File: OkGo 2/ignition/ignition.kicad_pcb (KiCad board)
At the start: 2 copper layers, 100 parts, among them K201 16A SPST, K202 16A SPST, K203 16A SPST, K204 16A SPST, K205 16A SPST, P105 BATT, P106 SMA, P107 ARM_LED, P109 BUZZ, P201 CH3_LED, P203 CH3, P204 CH1_LED, P206 CH1, P207 CH4_LED, P209 CH4, P210 CH2_LED, P212 CH2, Q101 BSS138BK, Q201 BSS138BK, Q202 BSS138BK, Q203 BSS138BK, Q204 BSS138BK, Q205 BSS138BK, U103 SWD, U105 RFM95W, U106 STM32F071CBT6, U107 TSR 0.5-2433, Y101 8MHz

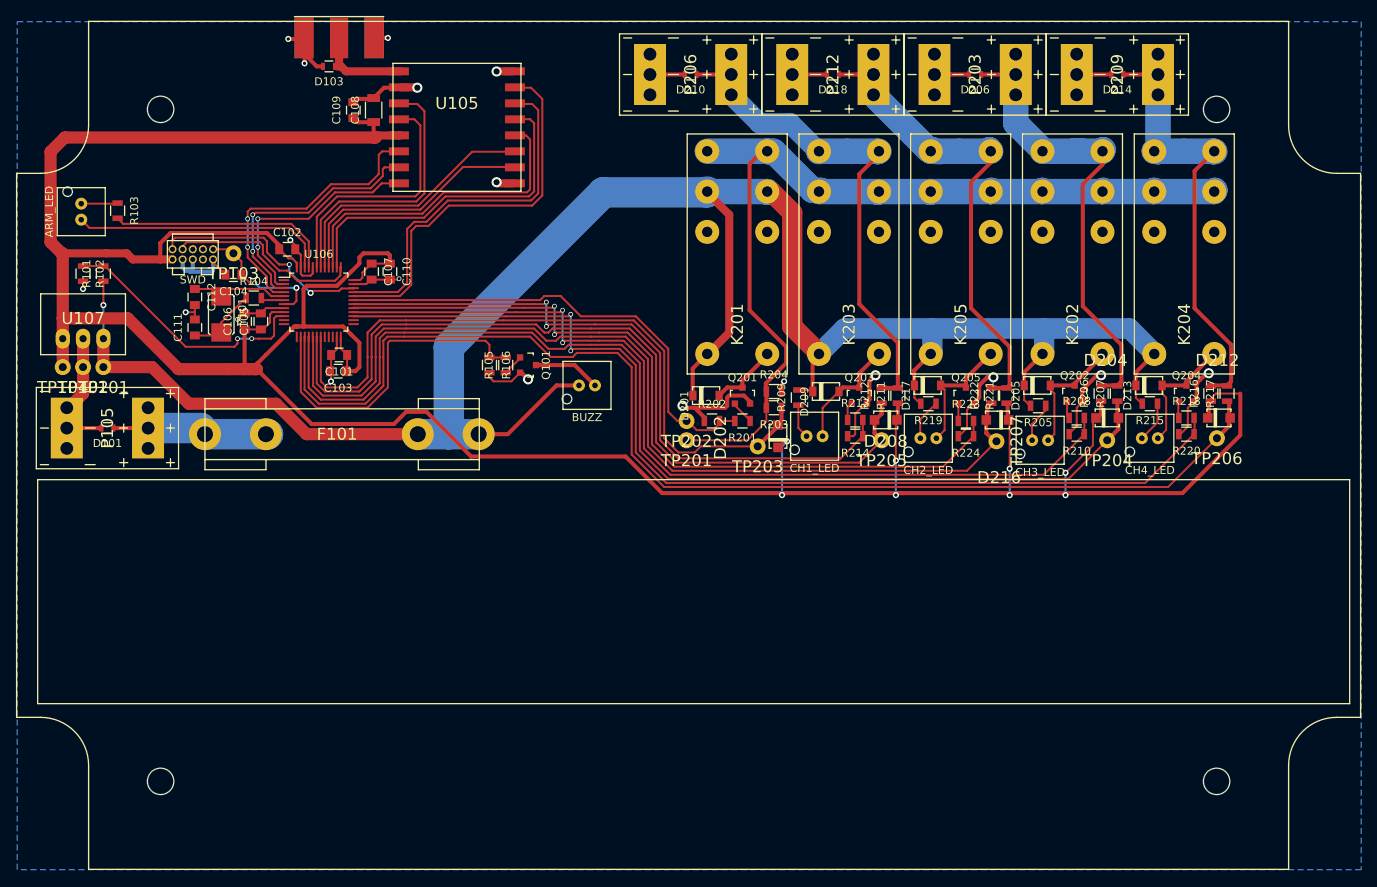
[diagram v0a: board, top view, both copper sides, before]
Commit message: Fixes #22
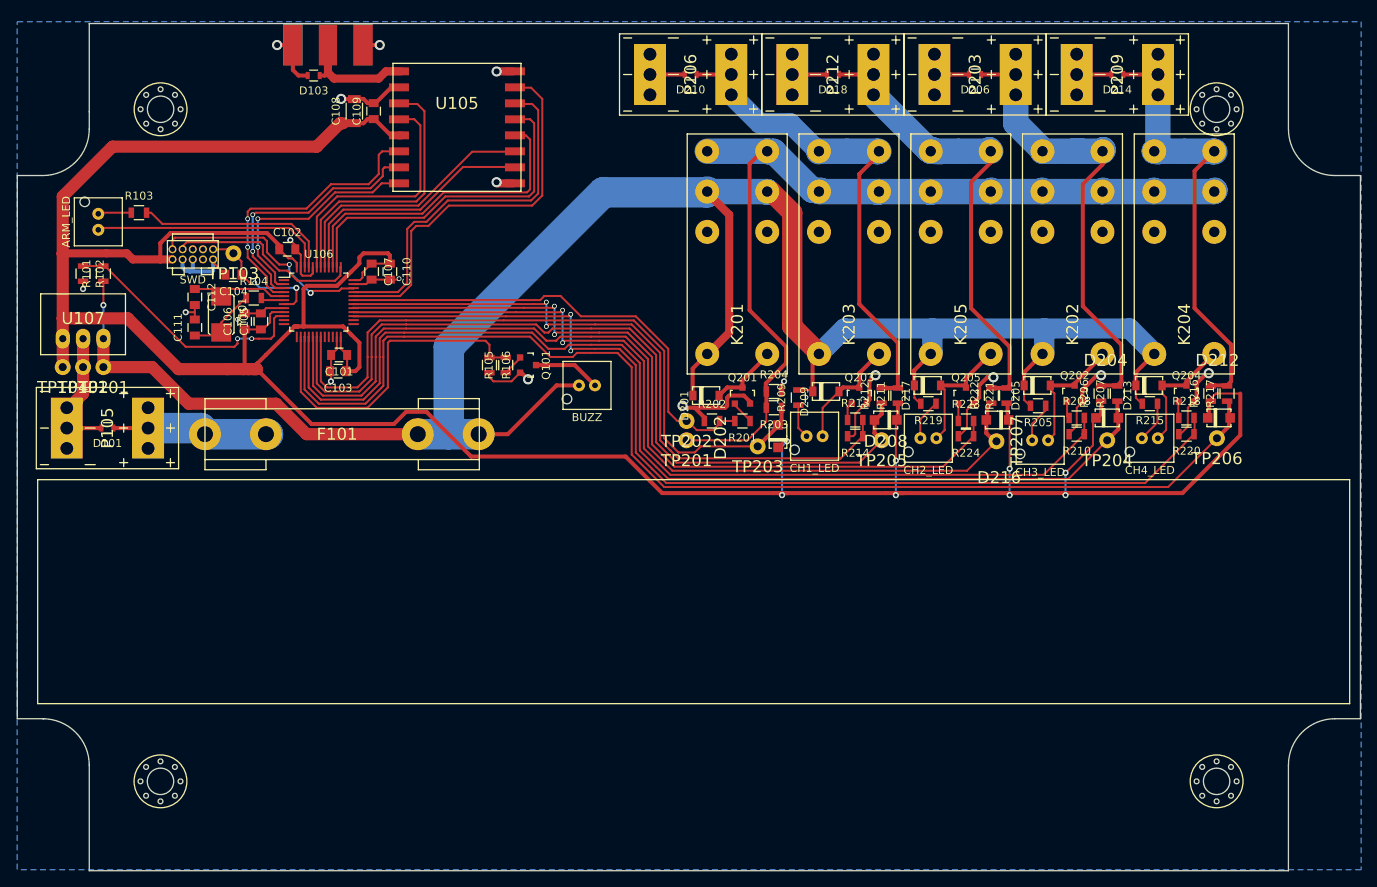
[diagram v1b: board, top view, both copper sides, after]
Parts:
- removed the REF** at (121.9, 101.7)
- added M3_MOUNT: VAL**, common:M3_MOUNT_FANCY, F.Cu at (55.9, 143.7)
- added M3_MOUNT: VAL**, common:M3_MOUNT_FANCY, F.Cu at (187.9, 143.7)
- added M3_MOUNT: VAL**, common:M3_MOUNT_FANCY, F.Cu at (187.9, 59.7)
- added M3_MOUNT: VAL**, common:M3_MOUNT_FANCY, F.Cu at (55.9, 59.7)
- moved R103 2.68 mm to (53.2, 72.6), turned to 0 degrees
- moved C109 2.54 mm to (82.5, 59.9)
- moved P107 2.48 mm to (48.1, 73.8)
- moved C108 2.42 mm to (80.1, 59.9)
- moved D103 2.22 mm to (75.1, 55.5)
- moved P106 1.66 mm to (76.8, 51.7)
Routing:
- net +3V3: track 401.4 -> 392.0 mm
- net /ARM_LED: track 28.4 -> 25.1 mm
- net GND: track 156.5 -> 153.8 mm, vias 19 -> 18
- net /DISARM_LED: track 32.2 -> 29.7 mm
- net Net-(P107-Pad2): track 4.82 -> 4.20 mm
- net Net-(D103-Pad1): track 13.9 -> 14.4 mm
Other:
- board outline added: 167.9 x 105.9 mm
